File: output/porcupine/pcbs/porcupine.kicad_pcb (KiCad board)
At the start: 2 copper layers, 140.5 x 103.1 mm, 54 parts, among them J1 Jumper, J2 Jumper

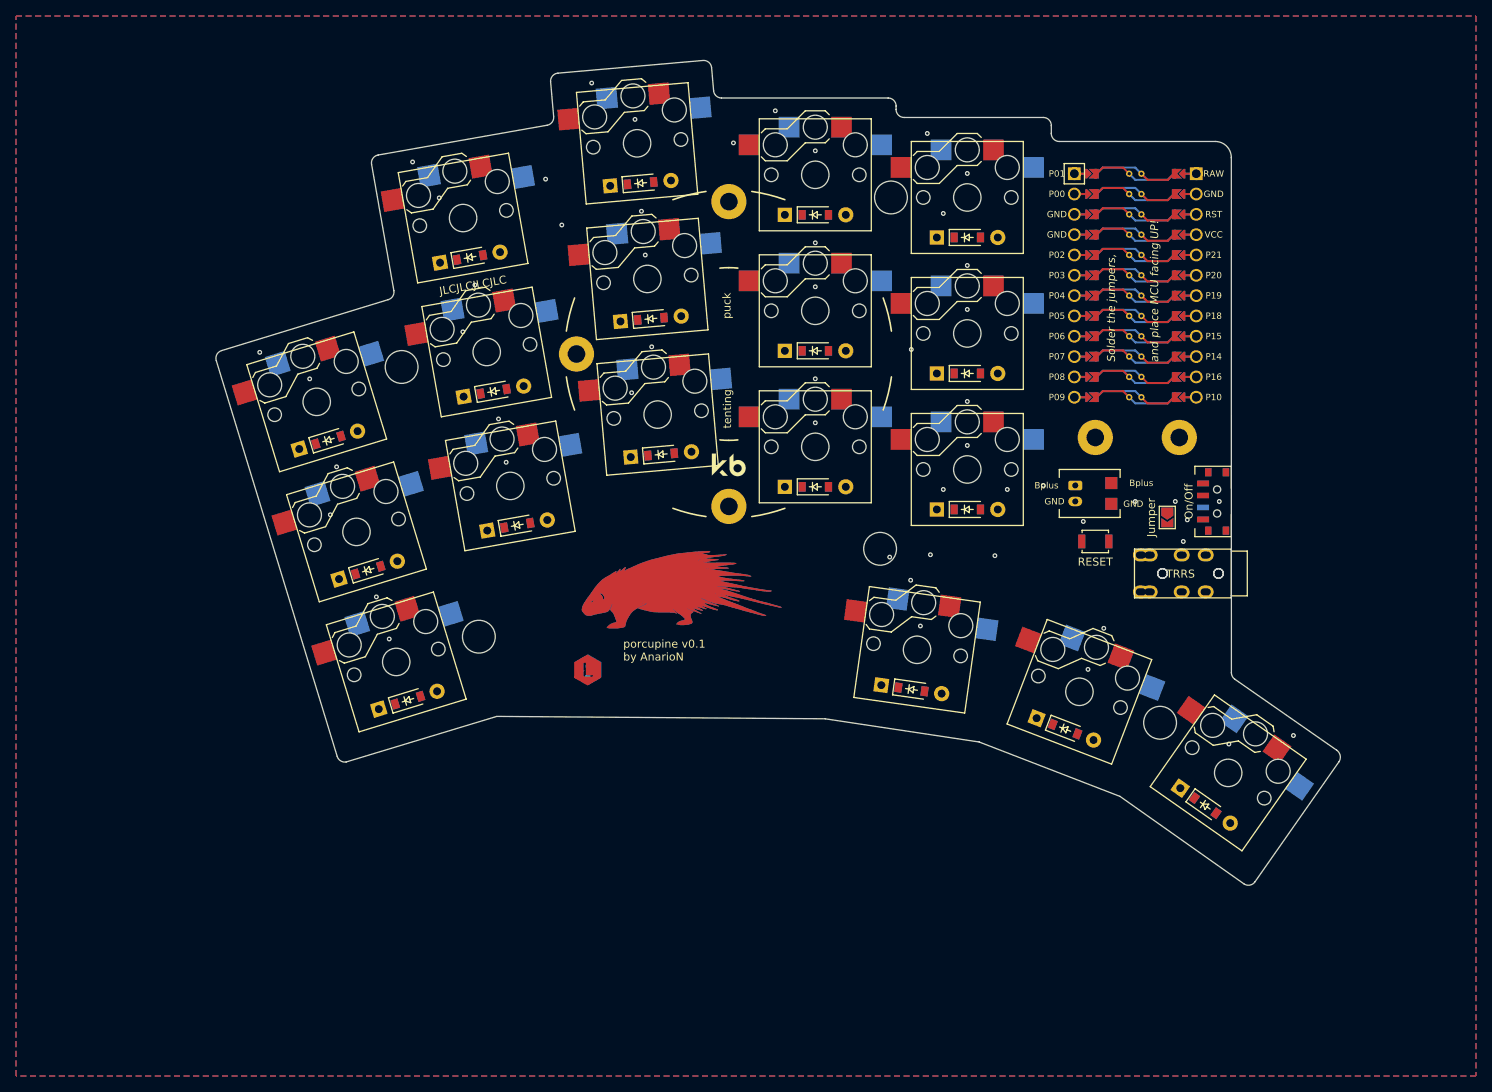
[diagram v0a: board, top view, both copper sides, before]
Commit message: Beschreibung deiner Änderungen
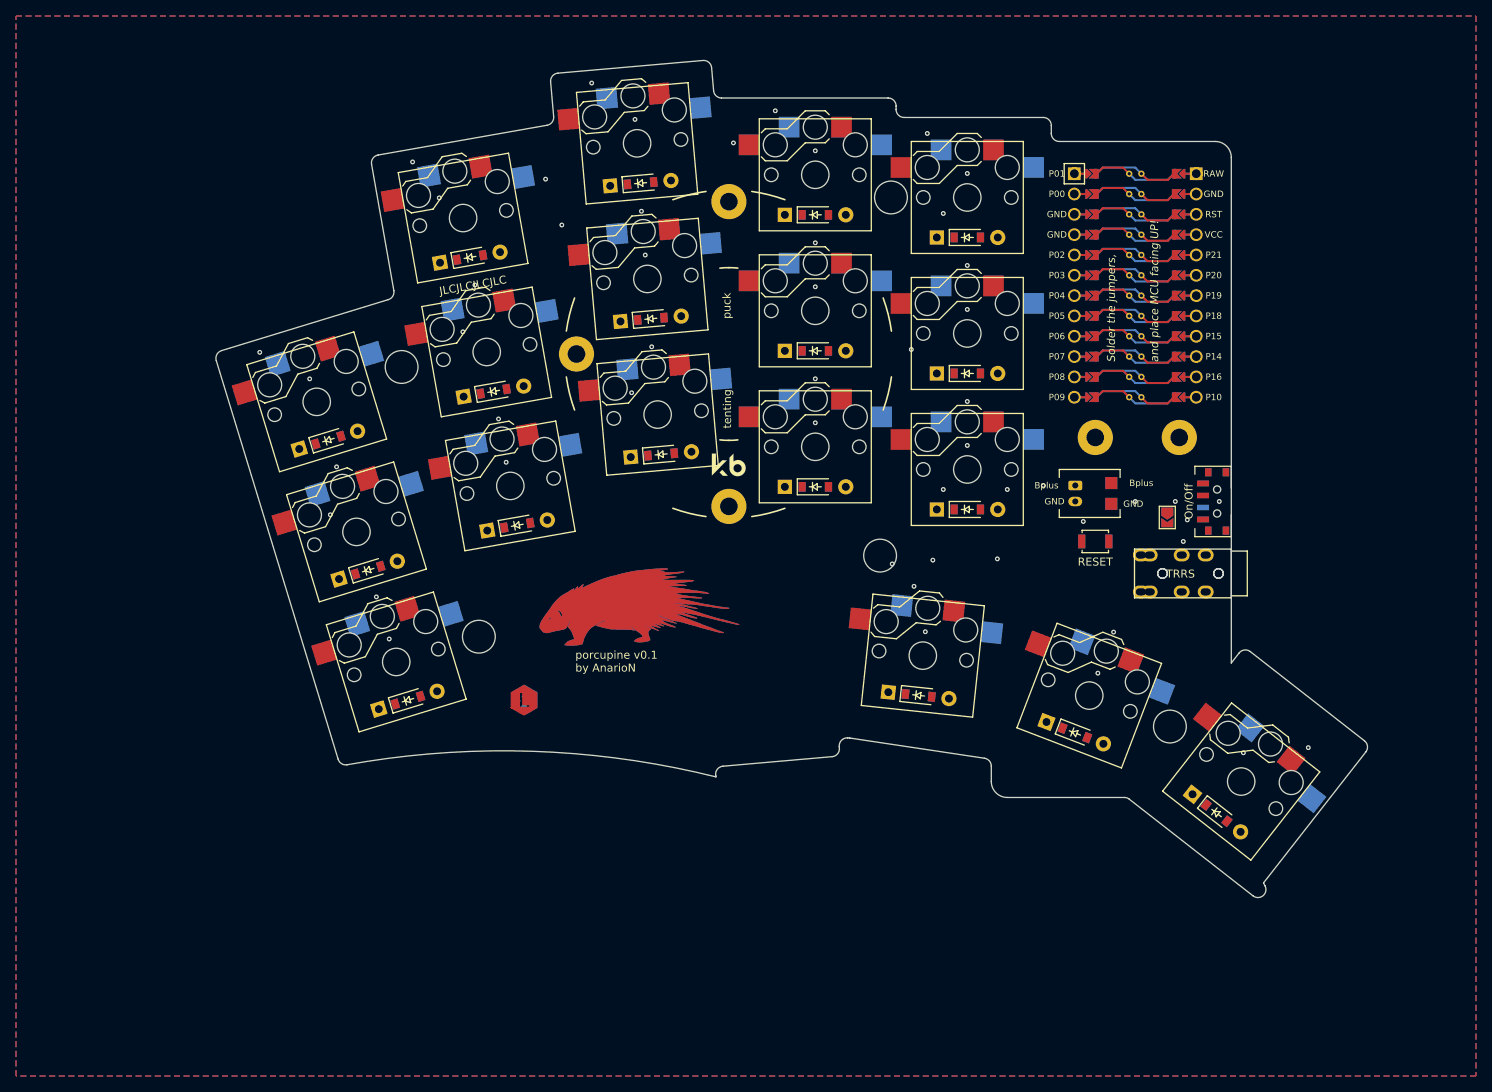
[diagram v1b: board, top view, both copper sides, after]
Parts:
- moved Side_B 8.80 mm to (189.6, 158.4)
- moved Side_F 8.80 mm to (189.6, 154.5)
- moved LOGO_B 5.71 mm to (205.4, 143.9)
- moved LOGO_F 5.71 mm to (205.4, 143.9)
- moved S18 1.95 mm to (280.7, 165.7), turned to -38 degrees
- moved D18 1.69 mm to (277.6, 169.6), turned to -38 degrees
- moved D17 1.32 mm to (259.9, 159.6)
- moved S17 1.32 mm to (261.7, 154.9)
- moved D16 1.17 mm to (240.3, 154.9), turned to -6 degrees
- moved S16 1.02 mm to (240.9, 150.0), turned to -6 degrees
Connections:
- D1 pad 2: pinky_bottom -> P6
- D10 pad 2: index_bottom -> P6
- D11 pad 2: index_home -> P5
- D12 pad 2: index_top -> P4
- D13 pad 2: inner_bottom -> P6
- D14 pad 2: inner_home -> P5
- D15 pad 2: inner_top -> P4
- D16 pad 2: near_thumb -> (no net)
- D17 pad 2: home_thumb -> (no net)
- D18 pad 2: far_thumb -> (no net)
- D2 pad 2: pinky_home -> P5
- D3 pad 2: pinky_top -> P4
- D4 pad 2: ring_bottom -> P6
- D5 pad 2: ring_home -> P5
- D6 pad 2: ring_top -> P4
- D7 pad 2: middle_bottom -> P6
- D8 pad 2: middle_home -> P5
- D9 pad 2: middle_top -> P4
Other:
- board size 140.5 x 103.1 mm -> 143.9 x 104.6 mm
- net class Default added: clearance 0.2, trace_width 0.25, via_dia 0.8, via_drill 0.4
- net class Power added: clearance 0.2, trace_width 0.5, via_dia 0.8, via_drill 0.4
